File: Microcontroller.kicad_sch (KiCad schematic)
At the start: 60 parts, among them J403 RJE721881411, J404 RJE721881411, U401 OwnTech_SPIN, U402 TCAN334GDR, U405 MAX33046EASA+T, U406 MCP6487T-E/SN

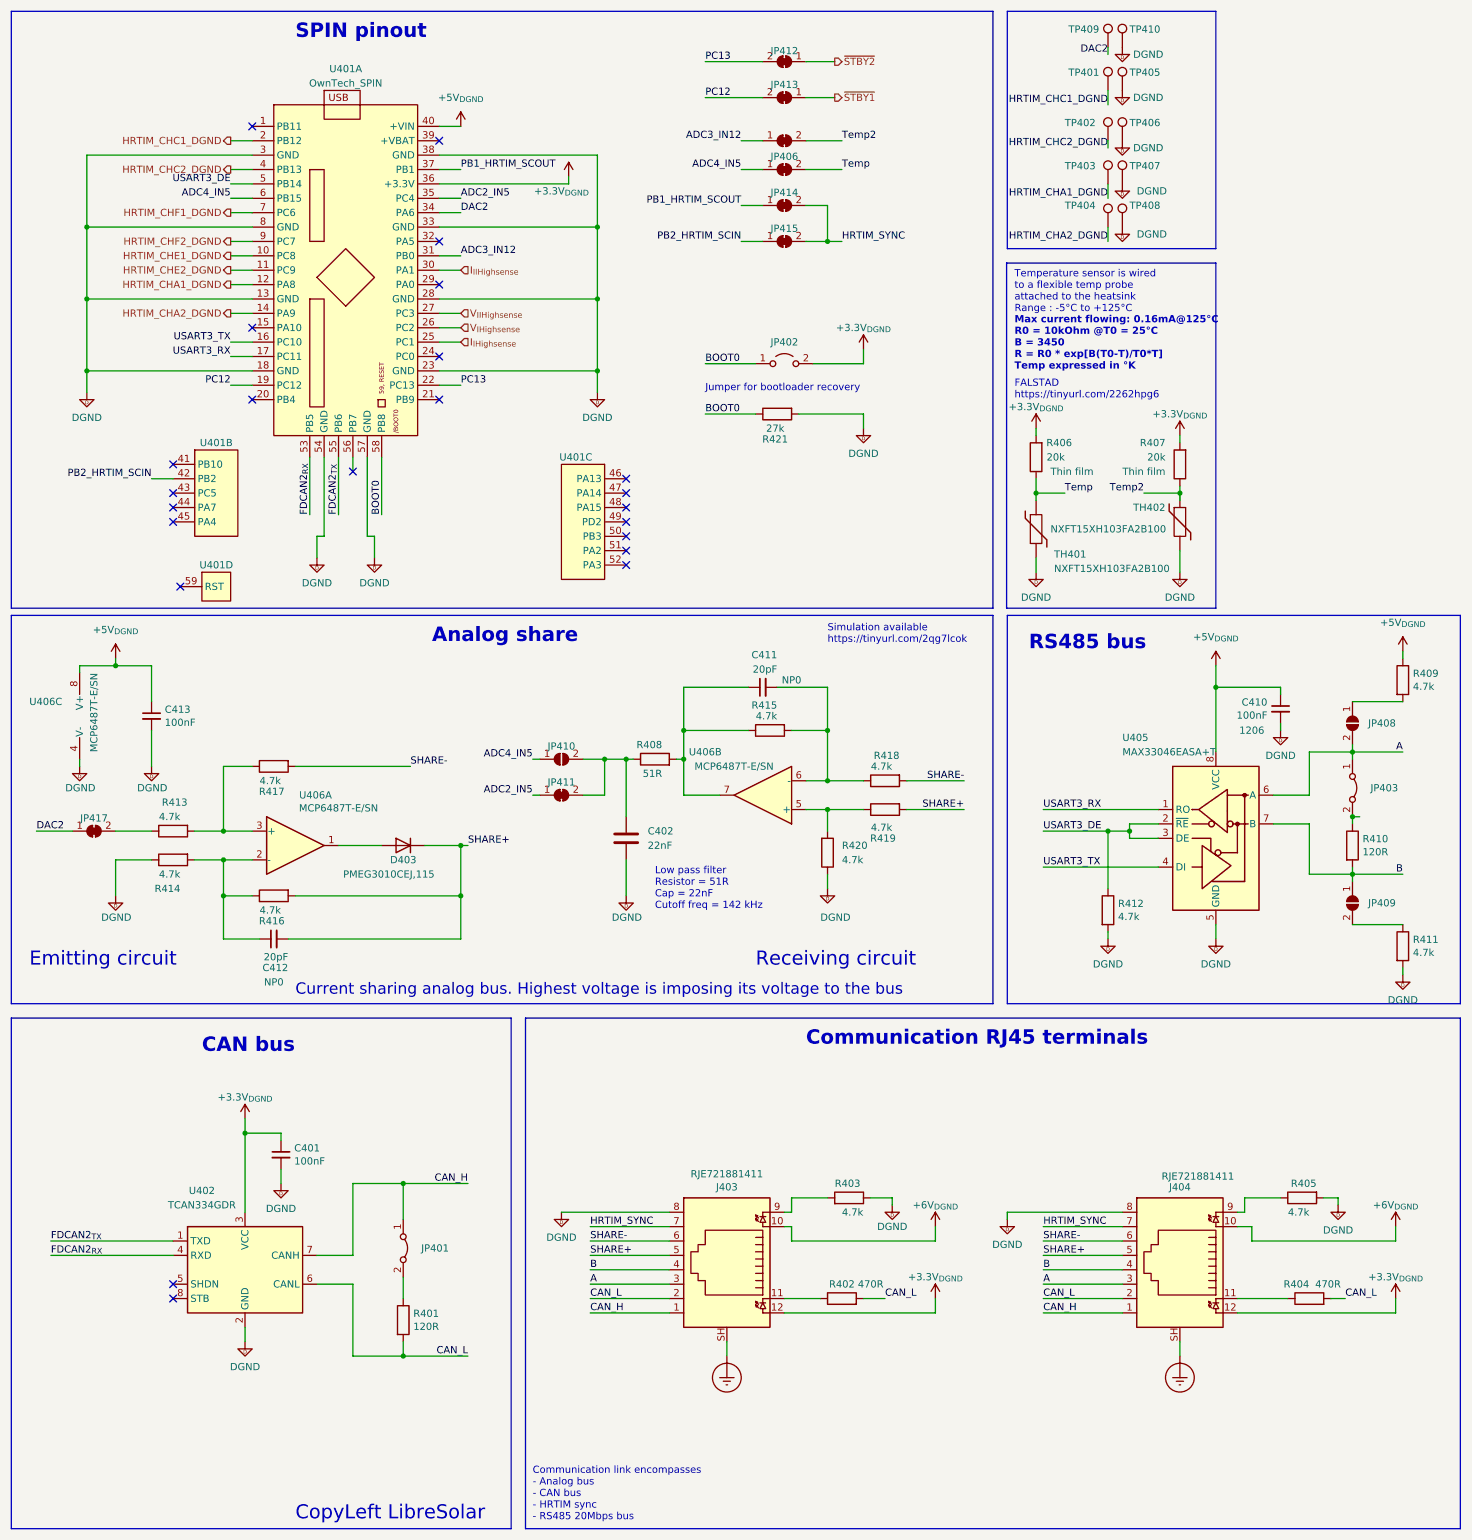
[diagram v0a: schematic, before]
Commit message: Initial commit micro-inverter
Signed-off-by: Jean Alinei <jean.alinei@owntech.org>
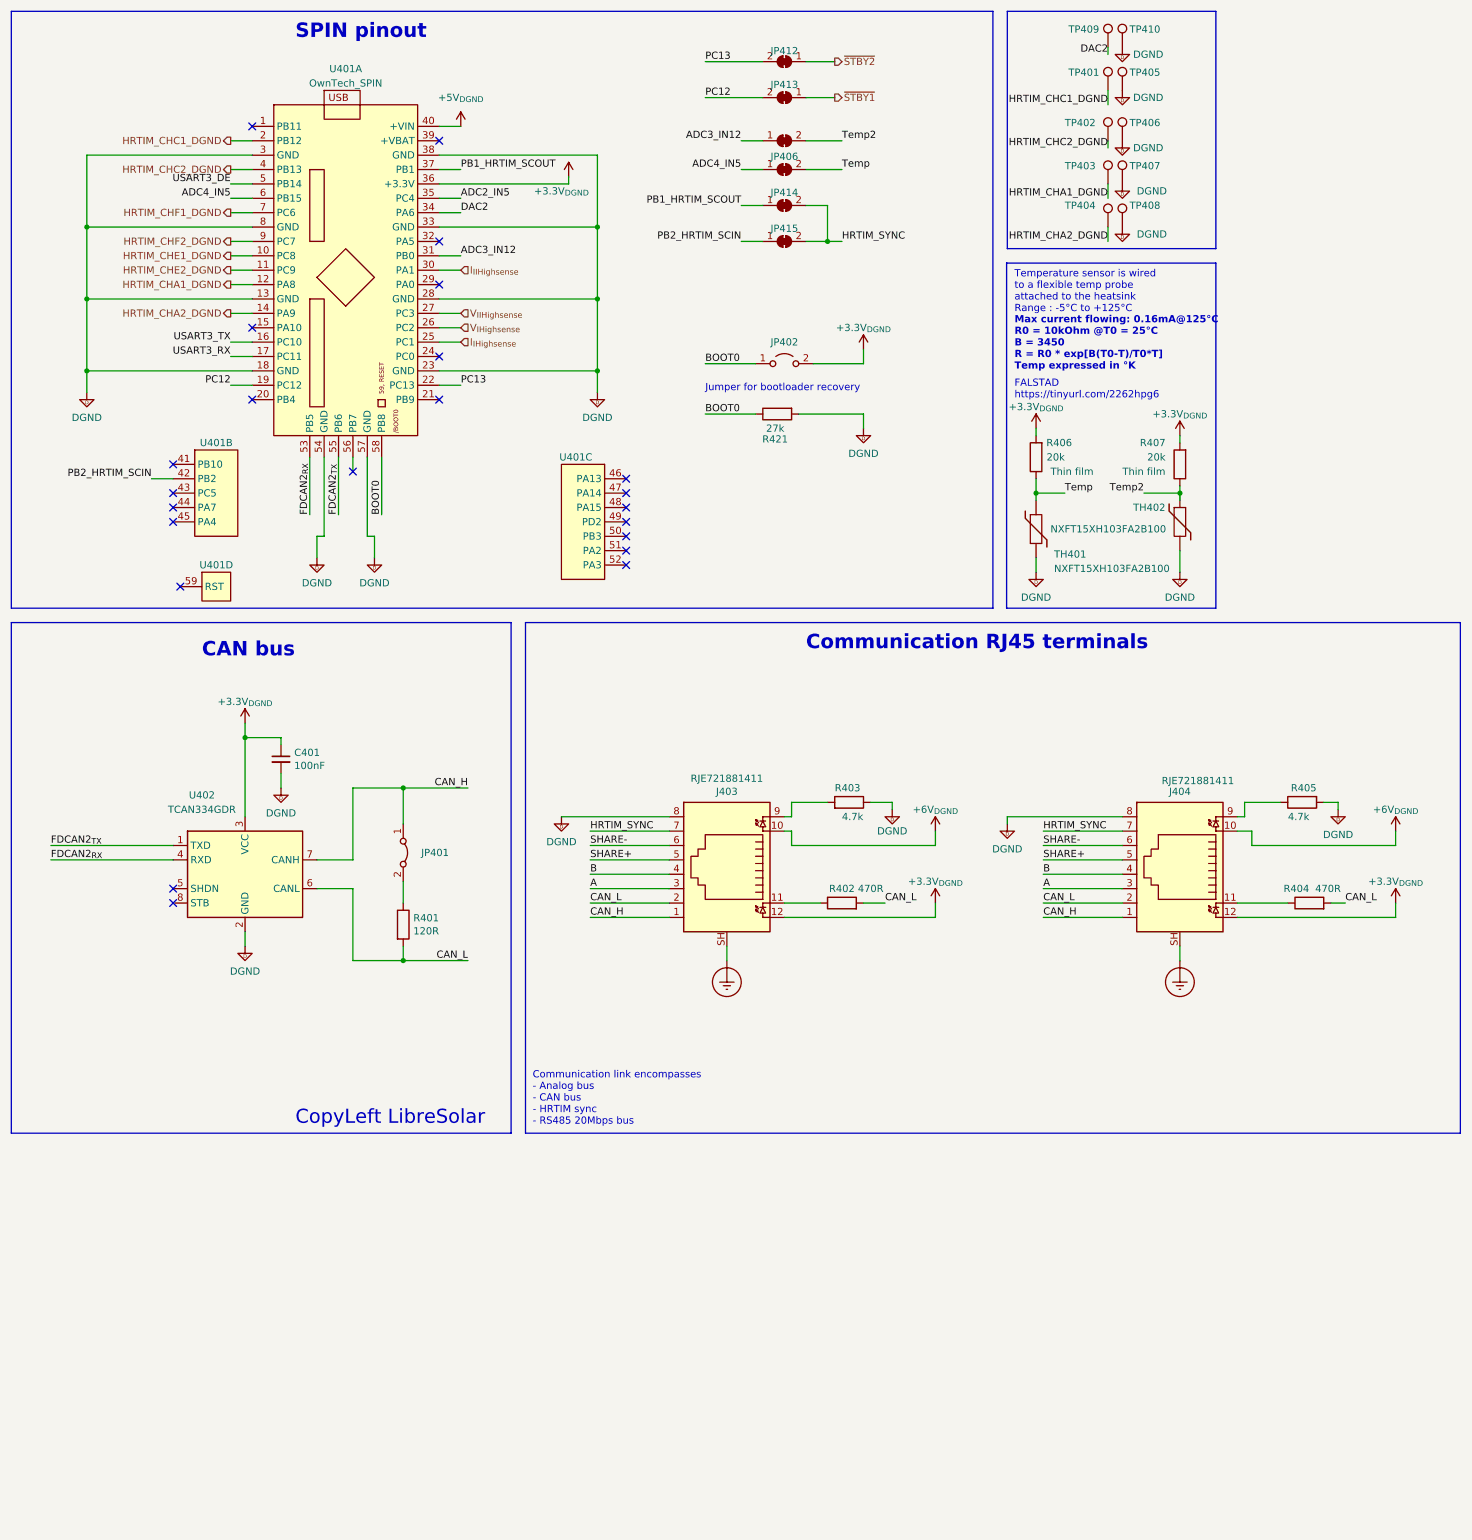
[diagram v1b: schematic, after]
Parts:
- removed C402: 22nF, Footprints:C_0805_2012Metric, symbol Device:C
- removed C410, C413: 100nF, Capacitor_SMD:C_1206_3216Metric, symbol Device:C_Small
- removed C411, C412: 20pF, Footprints:C_0805_2012Metric, symbol Device:C_Small
- removed D403: PMEG3010CEJ,115, Diode_SMD:D_SOD-323_HandSoldering, symbol Symbols:PMEG2010AEJ,115
- removed JP403: Jumper, Connector_PinHeader_2.54mm:PinHeader_1x02_P2.54mm_Vertical, symbol Jumper:Jumper_2_Bridged
- removed JP408, JP409: SolderJumper_2_Open, Jumper:SolderJumper-2_P1.3mm_Open_RoundedPad1.0x1.5mm, symbol Jumper:SolderJumper_2_Open
- removed JP410: Jumper_2_Bridged, Jumper:SolderJumper-2_P1.3mm_Open_RoundedPad1.0x1.5mm, symbol Jumper:SolderJumper_2_Open
- removed JP411, JP417: Jumper_2_Bridged, Jumper:SolderJumper-2_P1.3mm_Bridged_RoundedPad1.0x1.5mm, symbol Jumper:SolderJumper_2_Bridged
- removed R408: 51R, Footprints:R_0805_2012Metric, symbol Device:R
- removed R409, R411, R412, R413, R414, R415, R416, R417, R418, R419, R420: 4.7k, Footprints:R_0805_2012Metric, symbol Device:R
- removed R410: 120R, Footprints:R_0805_2012Metric, symbol Device:R
- removed U405: MAX33046EASA+T, Package_SO:SOIC-8_3.9x4.9mm_P1.27mm, symbol Interface_UART:LTC2850xS8
- removed U406: MCP6487T-E/SN, Package_SO:SOIC-8_3.9x4.9mm_P1.27mm, symbol Amplifier_Operational:OPA2277
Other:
- note removed: "Analog share"
- note removed: "Current sharing analog bus. Highest voltage is imposing its voltage to the bus"
- note removed: "Emitting circuit"
- note removed: "Low pass filter Resistor = 51R Cap = 22nF Cutoff freq = 142 kHz"
- note removed: "RS485 bus"
- note removed: "Receiving circuit"
- note removed: "Simulation available https://tinyurl.com/2qg7lcok"
- title: Microcontroller & Communication -> Micro-inverter - 400W
- moved on the sheet: C401, J403, J404, JP401, R401, R402, R403, R404, R405, U402
